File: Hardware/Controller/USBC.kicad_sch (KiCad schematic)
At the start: 12 parts, among them J301 USB_C_Receptacle_USB2.0_16P, Q301 Q_NMOS_GSD, U301 CH224K

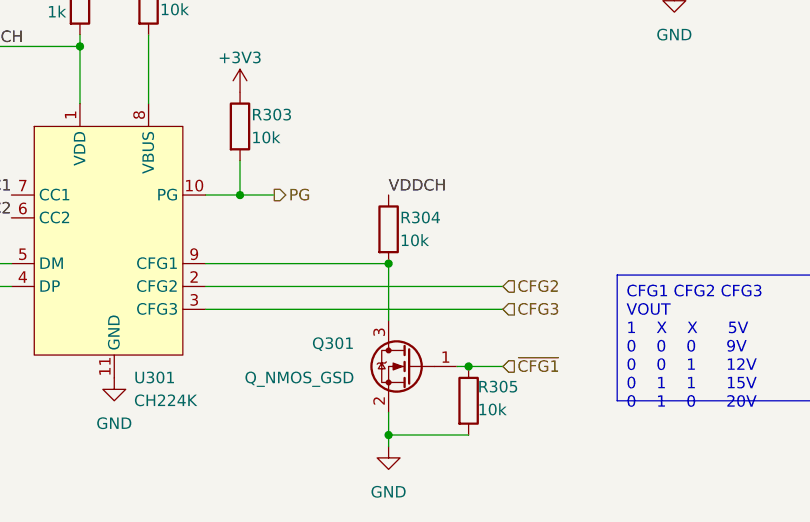
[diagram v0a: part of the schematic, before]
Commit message: Add software files
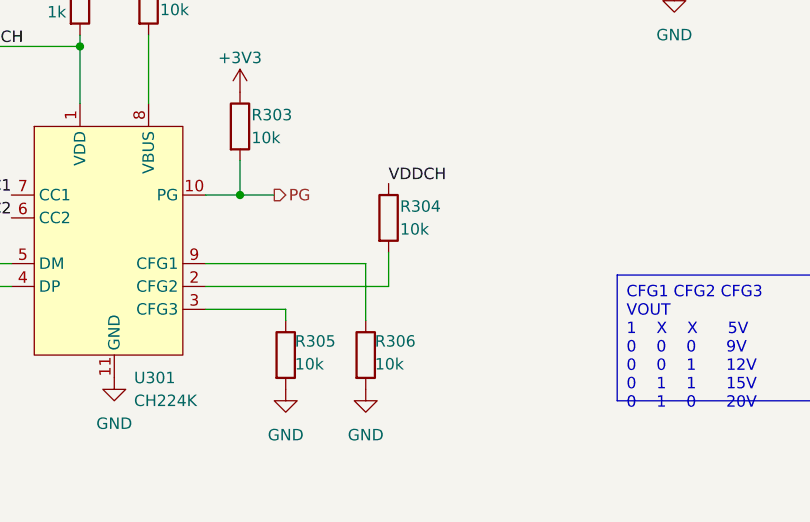
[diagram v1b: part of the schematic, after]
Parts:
- removed Q301: Q_NMOS_GSD, Package_TO_SOT_SMD:SOT-23-3, symbol Device:Q_NMOS_GSD
- added R306: 10k, Resistor_SMD:R_0402_1005Metric, symbol Device:R
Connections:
- net CFG2 is gone; now on an unnamed net: U301.2 (CFG2)
- net ~{CFG1} is gone; now on an unnamed net: R305.1
- net GND: now also R306.2
- net at R304.2: no longer U301.9 (CFG1)
- net CFG3: no longer names the net of U301.3 (CFG3)
- new net: R306.1, U301.9 (CFG1)
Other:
- moved on the sheet: R304
